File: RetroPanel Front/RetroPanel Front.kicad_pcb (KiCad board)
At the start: 2 copper layers, 100 x 22.5 mm, 18 parts, among them J1 Front Panel, M1 Mounting_Pin, M10 Mounting_Pad, M2 Mounting_Pin, M3 Mounting_Pin, M4 Mounting_Pin, M5 Mounting_Pad, M6 Mounting_Pad, M7 Mounting_Pad, M8 Mounting_Pad, M9 Mounting_Pad, SW1 TURBO, SW2 POWER, SW3 RESET, SW4 EXTRA, U1 3641AH

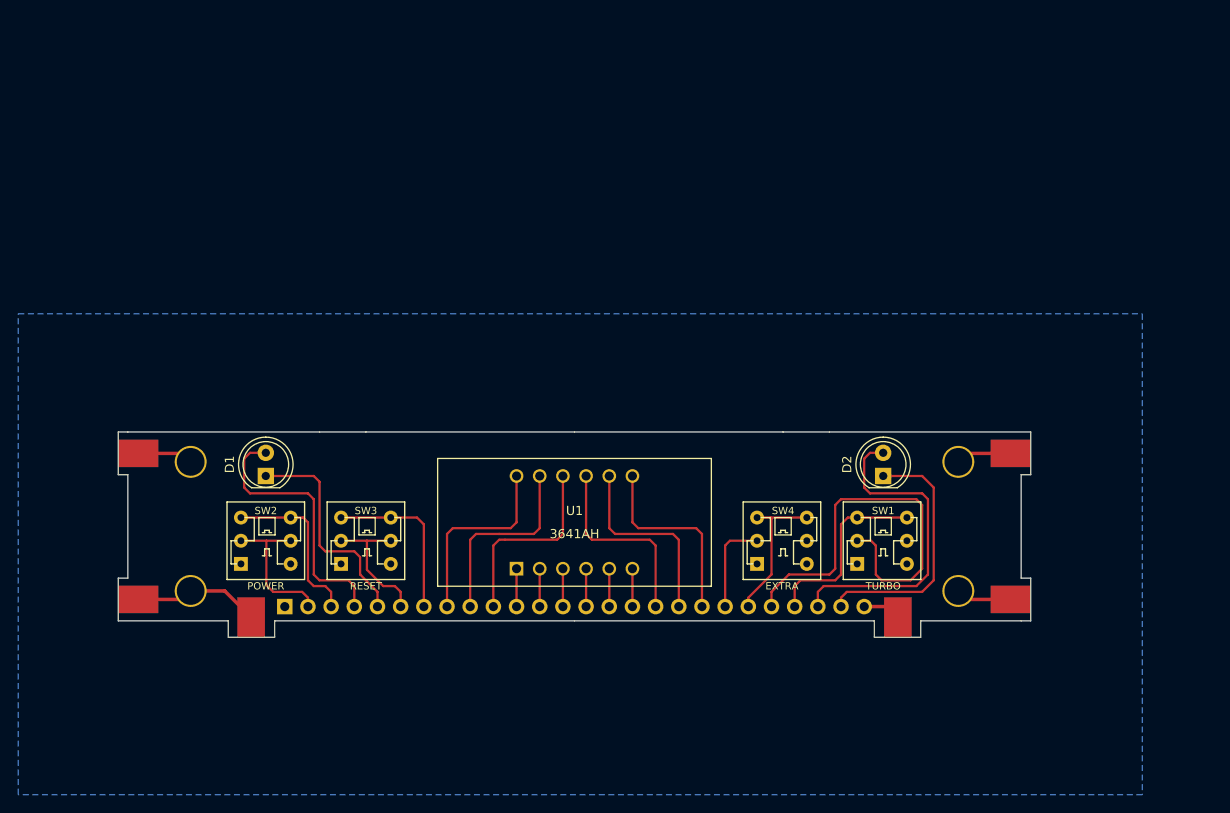
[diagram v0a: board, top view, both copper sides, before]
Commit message: Match grid
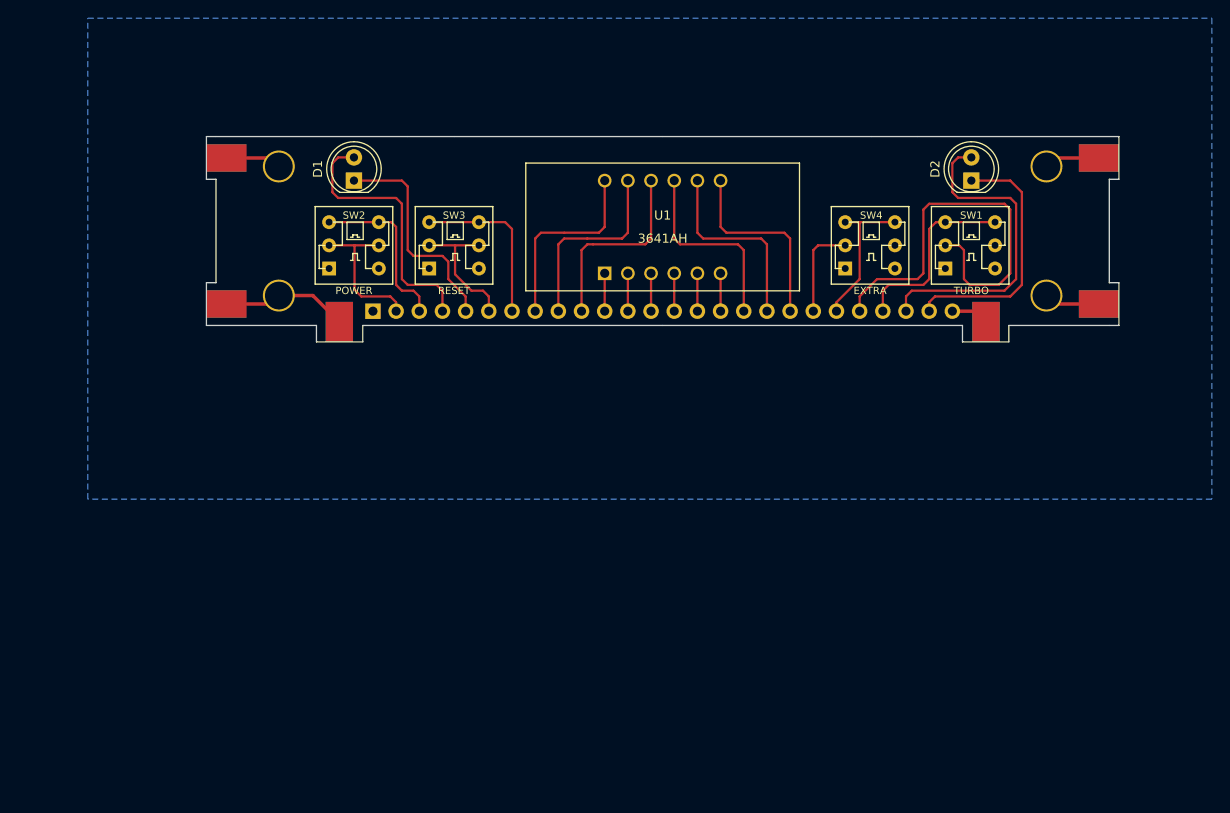
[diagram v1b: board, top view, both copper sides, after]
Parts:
- moved D2 33.8 mm to (184.6, 84.1)
- moved D1 33.8 mm to (116.9, 84.1)
- moved J1 33.8 mm to (119.0, 98.4)
- moved M1 33.8 mm to (108.7, 96.7)
- moved M10 33.8 mm to (198.6, 97.7)
- moved M2 33.8 mm to (192.8, 96.7)
- moved M3 33.8 mm to (192.8, 82.6)
- moved M4 33.8 mm to (108.7, 82.6)
- moved M5 33.8 mm to (102.9, 81.6)
- moved M6 33.8 mm to (186.2, 99.6)
- moved M7 33.8 mm to (102.9, 97.7)
- moved M8 33.8 mm to (115.3, 99.6)
- moved M9 33.8 mm to (198.6, 81.6)
- moved SW1 33.8 mm to (184.5, 91.2)
- moved SW2 33.8 mm to (116.9, 91.2)
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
